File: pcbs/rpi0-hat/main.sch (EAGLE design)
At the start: 10 parts, among them IC1 MCP23017SP2, IC2 MCP3008

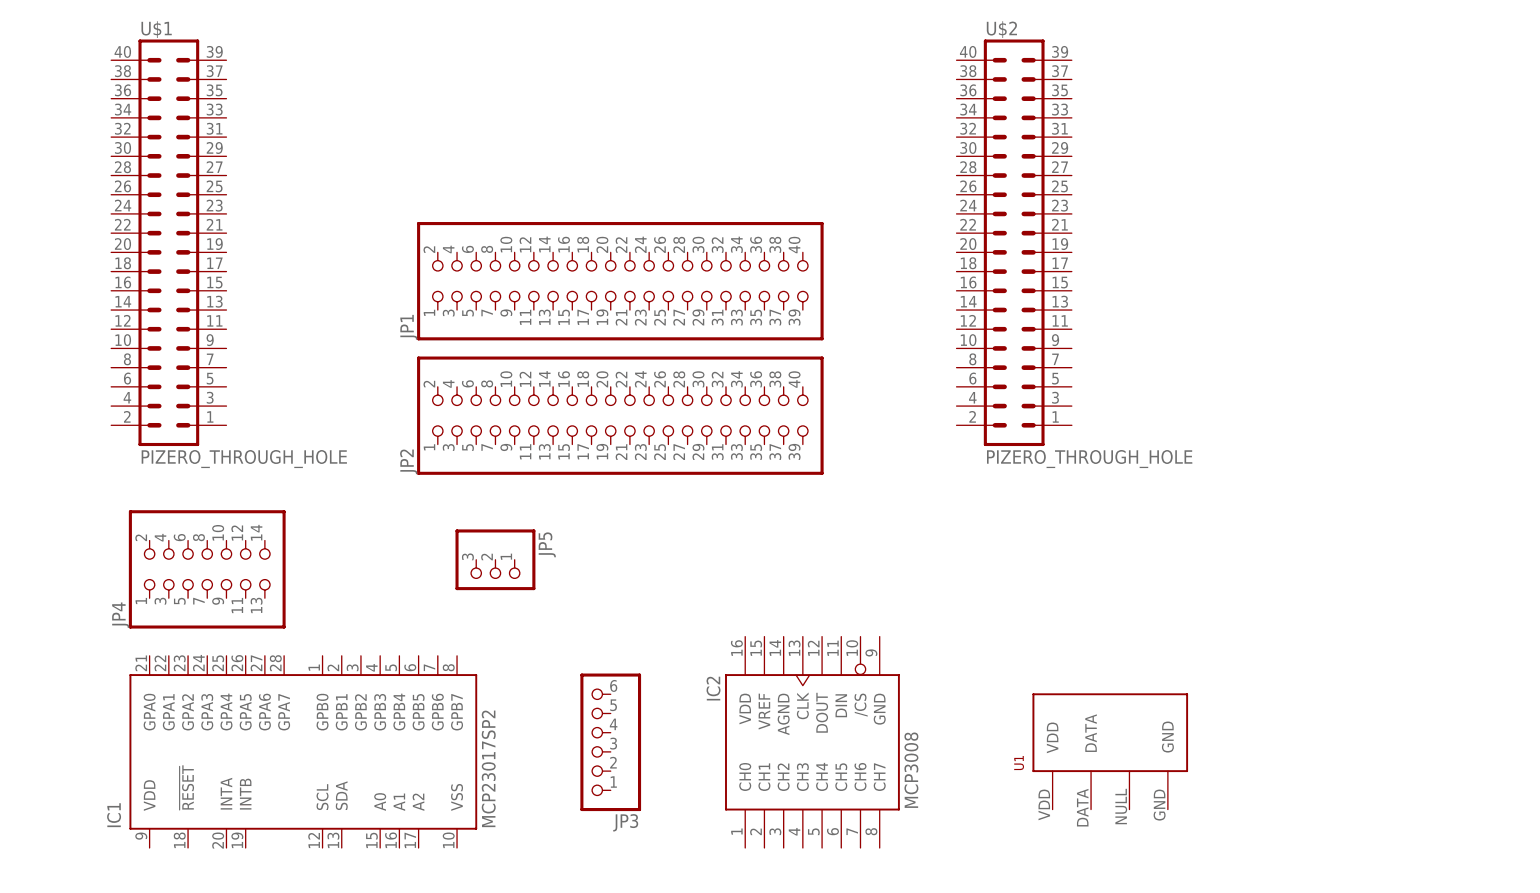
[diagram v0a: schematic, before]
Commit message: significant time change forecast
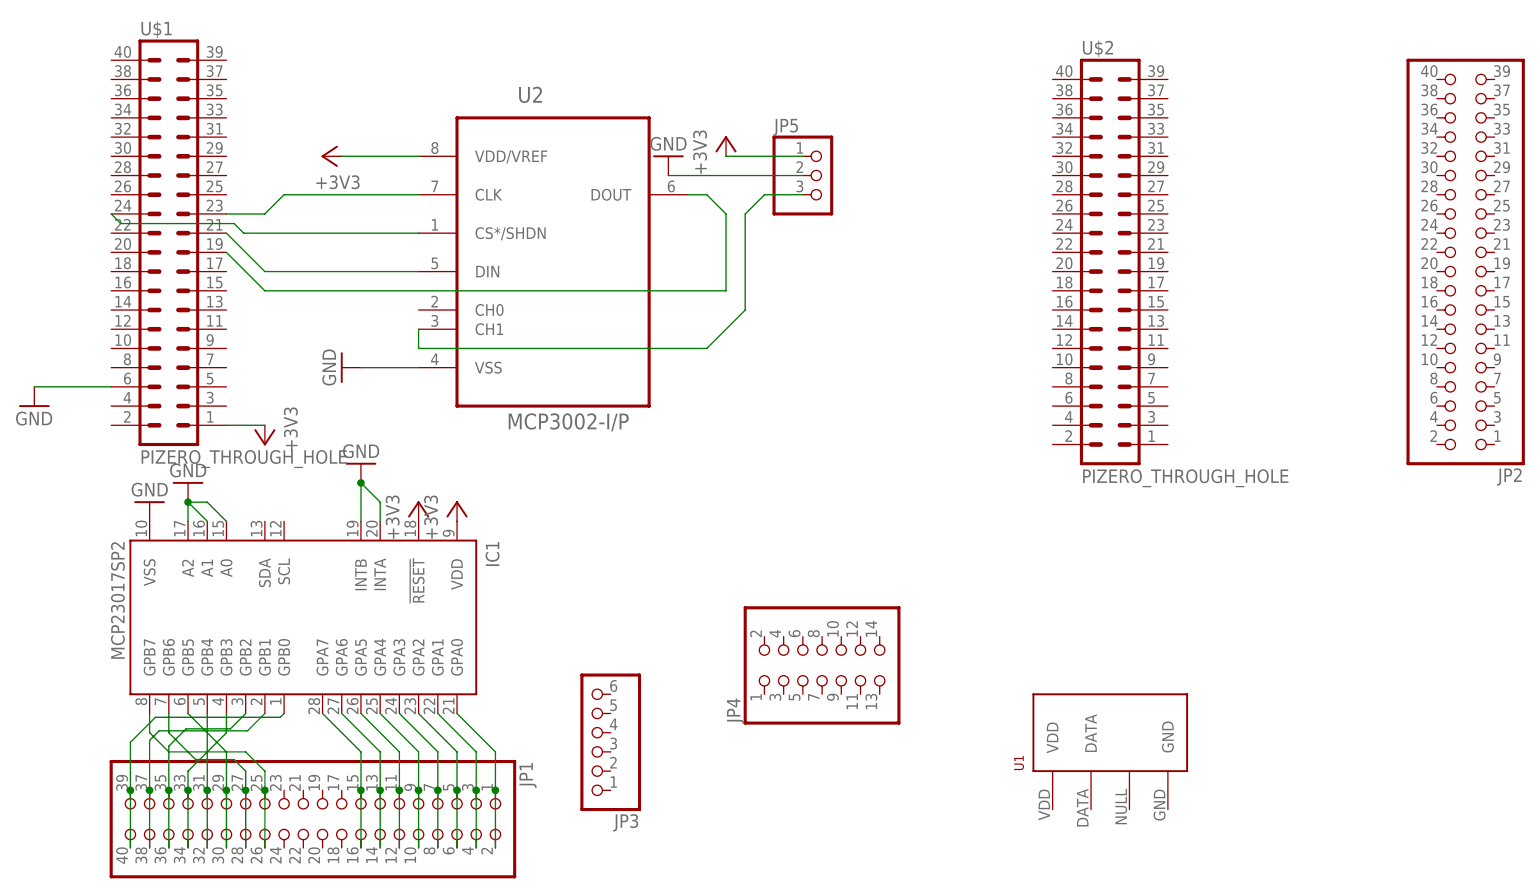
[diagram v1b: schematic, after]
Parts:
- removed IC2: MCP3008, adafruit:MCP3008
- added U2: MCP3002-I/P, mcp:MCP3002-I/P
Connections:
- new net +3V3: IC1.!RESET, IC1.VDD, JP5.1, U$1.1, U2.VDD/VREF
- new net GND: IC1.A0, IC1.A1, IC1.A2, IC1.INTA, IC1.INTB, IC1.VSS, JP5.2, U$1.6, U2.VSS
- new net N$1: U$1.24, U2.CS*/SHDN
- new net N$10: IC1.GPB3, JP1.33, JP1.34
- new net N$11: IC1.GPB4, JP1.31, JP1.32
- new net N$12: IC1.GPB5, JP1.29, JP1.30
- new net N$13: IC1.GPB6, JP1.27, JP1.28
- new net N$14: IC1.GPB7, JP1.25, JP1.26
- new net N$15: IC1.GPA0, JP1.1, JP1.2
- new net N$16: IC1.GPA1, JP1.3, JP1.4
- new net N$17: IC1.GPA2, JP1.5, JP1.6
- new net N$18: IC1.GPA3, JP1.7, JP1.8
- new net N$19: IC1.GPA4, JP1.10, JP1.9
- new net N$2: U$1.23, U2.CLK
- new net N$20: IC1.GPA5, JP1.11, JP1.12
- new net N$21: IC1.GPA6, JP1.13, JP1.14
- new net N$22: IC1.GPA7, JP1.15, JP1.16
- new net N$3: U$1.21, U2.DIN
- new net N$4: JP5.3, U2.CH1
- new net N$5: U$1.19, U2.DOUT
- new net N$7: IC1.GPB0, JP1.39, JP1.40
- new net N$8: IC1.GPB1, JP1.37, JP1.38
- new net N$9: IC1.GPB2, JP1.35, JP1.36
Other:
- moved on the sheet: IC1, JP1, JP2, JP4, JP5, U$2
